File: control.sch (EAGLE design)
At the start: 110 parts, among them IC1 LM358N, IC2 XMEGA16A4A, IC3 LM317MBSTT3, IC5 LM358N, Q1 BSS123, Q10 TIP42C, Q11 BC338, Q12 BC548, Q13 BC557C, Q14 BSS123, Q15 BSS123, Q16 BSS123, Q2 BSS123, Q3 BC548, Q4 BC557C, Q5 TIP41C, Q6 TIP42C, Q7 BC338, Q8 BSS123, Q9 TIP41C, X1 250-202/000-002, X3 250-204, X6 250-204

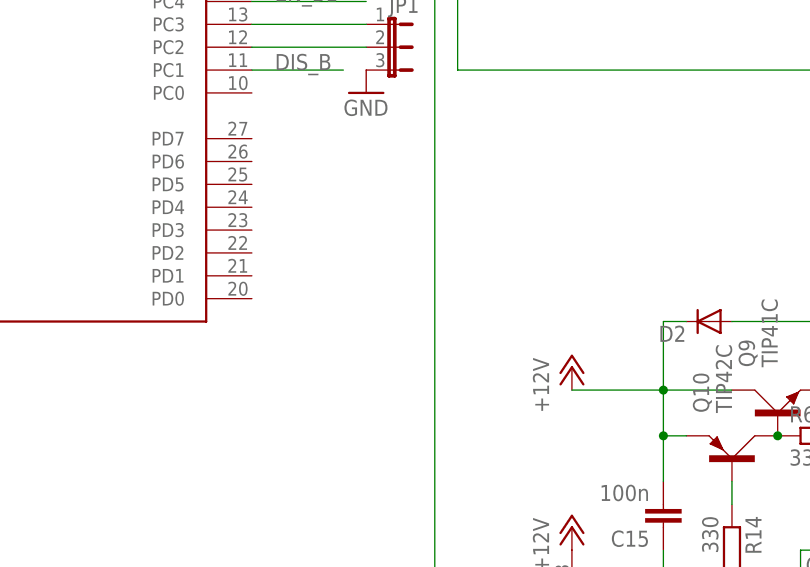
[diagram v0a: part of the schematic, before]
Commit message: LEDs
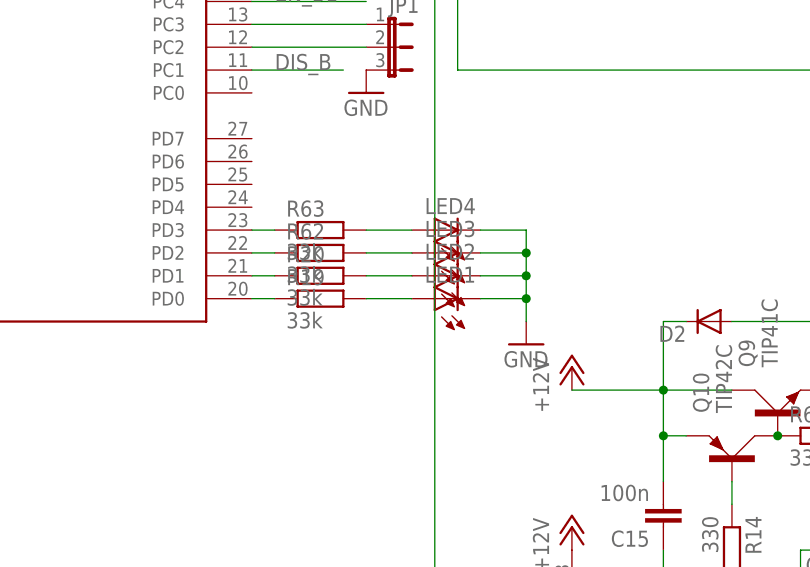
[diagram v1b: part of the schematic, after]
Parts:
- added LED1, LED2, LED3, LED4: (no value), led:LEDCHIPLED_0805
- added R19, R20, R62, R63: 33k, resistor:R-EU_M0805
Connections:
- new net N$10: IC2.PD1, R20.1
- new net N$39: IC2.PD2, R62.1
- new net N$5: IC2.PD0, R19.1
- new net N$58: IC2.PD3, R63.1
- new net N$59: LED4.A, R63.2
- new net N$60: LED3.A, R62.2
- new net N$61: LED2.A, R20.2
- new net N$62: LED1.A, R19.2
- net GND: now also LED1.C, LED2.C, LED3.C, LED4.C
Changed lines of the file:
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@@
 <part name="JP1" library="jumper" deviceset="JP2E" device=""/>
 <part name="GND23" library="supply1" deviceset="GND" device=""/>
+<part name="LED1" library="led" deviceset="LED" device="CHIPLED_0805"/>
+<part name="LED2" library="led" deviceset="LED" device="CHIPLED_0805"/>
+<part name="LED3" library="led" deviceset="LED" device="CHIPLED_0805"/>
+<part name="LED4" library="led" deviceset="LED" device="CHIPLED_0805"/>
+<part name="R19" library="resistor" deviceset="R-EU_" device="M0805" value="33k"/>
+<part name="R20" library="resistor" deviceset="R-EU_" device="M0805" value="33k"/>
+<part name="R62" library="resistor" deviceset="R-EU_" device="M0805" value="33k"/>
+<part name="R63" library="resistor" deviceset="R-EU_" device="M0805" value="33k"/>
+<part name="GND9" library="supply1" deviceset="GND" device=""/>
 </parts>
 <sheets>
@@
 <instance part="JP1" gate="1" x="172.72" y="187.96" rot="R270"/>
 <instance part="GND23" gate="1" x="170.18" y="182.88"/>
+<instance part="LED1" gate="G$1" x="177.8" y="160.02" rot="R90"/>
+<instance part="LED2" gate="G$1" x="177.8" y="162.56" rot="R90"/>
+<instance part="LED3" gate="G$1" x="177.8" y="165.1" rot="R90"/>
+<instance part="LED4" gate="G$1" x="177.8" y="167.64" rot="R90"/>
+<instance part="R19" gate="G$1" x="165.1" y="160.02"/>
+<instance part="R20" gate="G$1" x="165.1" y="162.56"/>
+<instance part="R62" gate="G$1" x="165.1" y="165.1"/>
+<instance part="R63" gate="G$1" x="165.1" y="167.64"/>
+<instance part="GND9" gate="1" x="187.96" y="154.94"/>
 </instances>
 <busses>
@@
 <pinref part="JP1" gate="1" pin="3"/>
 <pinref part="GND23" gate="1" pin="GND"/>
+</segment>
+<segment>
+<pinref part="GND9" gate="1" pin="GND"/>
+<wire x1="187.96" y1="167.64" x2="187.96" y2="165.1" width="0.1524" layer="91"/>
+<pinref part="LED1" gate="G$1" pin="C"/>
+<wire x1="187.96" y1="165.1" x2="187.96" y2="162.56" width="0.1524" layer="91"/>
+<wire x1="187.96" y1="162.56" x2="187.96" y2="160.02" width="0.1524" layer="91"/>
+<wire x1="187.96" y1="160.02" x2="187.96" y2="157.48" width="0.1524" layer="91"/>
+<wire x1="182.88" y1="160.02" x2="187.96" y2="160.02" width="0.1524" layer="91"/>
+<junction x="187.96" y="160.02"/>
+<pinref part="LED2" gate="G$1" pin="C"/>
+<wire x1="187.96" y1="162.56" x2="182.88" y2="162.56" width="0.1524" layer="91"/>
+<junction x="187.96" y="162.56"/>
+<pinref part="LED3" gate="G$1" pin="C"/>
+<wire x1="182.88" y1="165.1" x2="187.96" y2="165.1" width="0.1524" layer="91"/>
+<junction x="187.96" y="165.1"/>
+<pinref part="LED4" gate="G$1" pin="C"/>
+<wire x1="187.96" y1="167.64" x2="182.88" y2="167.64" width="0.1524" layer="91"/>
 </segment>
 </net>
@@
 </segment>
 </net>
+<net name="N$5" class="0">
+<segment>
+<pinref part="IC2" gate="G$1" pin="PD0"/>
+<pinref part="R19" gate="G$1" pin="1"/>
+<wire x1="160.02" y1="160.02" x2="157.48" y2="160.02" width="0.1524" layer="91"/>
+</segment>
+</net>
+<net name="N$10" class="0">
+<segment>
+<pinref part="IC2" gate="G$1" pin="PD1"/>
+<pinref part="R20" gate="G$1" pin="1"/>
+<wire x1="160.02" y1="162.56" x2="157.48" y2="162.56" width="0.1524" layer="91"/>
+</segment>
+</net>
+<net name="N$39" class="0">
+<segment>
+<pinref part="IC2" gate="G$1" pin="PD2"/>
+<pinref part="R62" gate="G$1" pin="1"/>
+<wire x1="160.02" y1="165.1" x2="157.48" y2="165.1" width="0.1524" layer="91"/>
+</segment>
+</net>
+<net name="N$58" class="0">
+<segment>
+<pinref part="IC2" gate="G$1" pin="PD3"/>
+<pinref part="R63" gate="G$1" pin="1"/>
+<wire x1="160.02" y1="167.64" x2="157.48" y2="167.64" width="0.1524" layer="91"/>
+</segment>
+</net>
+<net name="N$59" class="0">
+<segment>
+<pinref part="R63" gate="G$1" pin="2"/>
+<pinref part="LED4" gate="G$1" pin="A"/>
+<wire x1="170.18" y1="167.64" x2="175.26" y2="167.64" width="0.1524" layer="91"/>
+</segment>
+</net>
+<net name="N$60" class="0">
+<segment>
+<pinref part="LED3" gate="G$1" pin="A"/>
+<pinref part="R62" gate="G$1" pin="2"/>
+<wire x1="175.26" y1="165.1" x2="170.18" y2="165.1" width="0.1524" layer="91"/>
+</segment>
+</net>
+<net name="N$61" class="0">
+<segment>
+<pinref part="R20" gate="G$1" pin="2"/>
+<pinref part="LED2" gate="G$1" pin="A"/>
+<wire x1="170.18" y1="162.56" x2="175.26" y2="162.56" width="0.1524" layer="91"/>
+</segment>
+</net>
+<net name="N$62" class="0">
+<segment>
+<pinref part="LED1" gate="G$1" pin="A"/>
+<pinref part="R19" gate="G$1" pin="2"/>
+<wire x1="175.26" y1="160.02" x2="170.18" y2="160.02" width="0.1524" layer="91"/>
+</segment>
+</net>
